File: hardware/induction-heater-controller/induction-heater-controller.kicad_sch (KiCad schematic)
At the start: 21 parts, among them IC1 THVD1449DR, J1 Conn_ARM_SWD_TagConnect_TC203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, J1 RJ12, J2 Screw_Terminal_01x02, SW1 SW_Push, SW3 SW_Push, U1 STM32G030F6Px, U2 NCP718xSN330

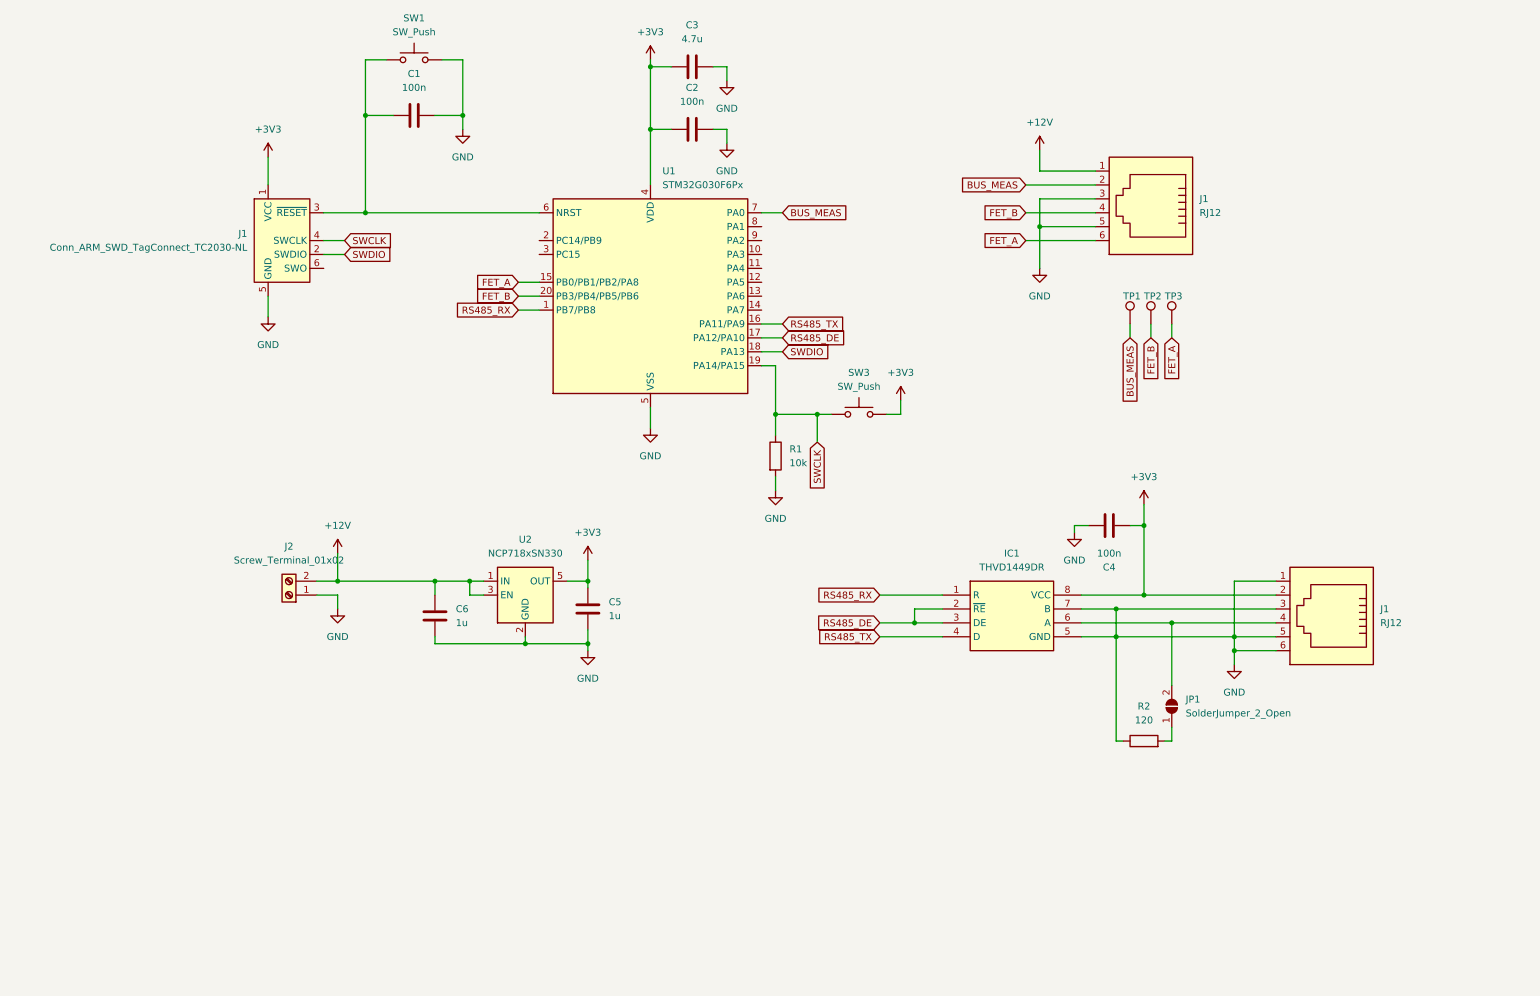
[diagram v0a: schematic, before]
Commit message: Finished board for controller
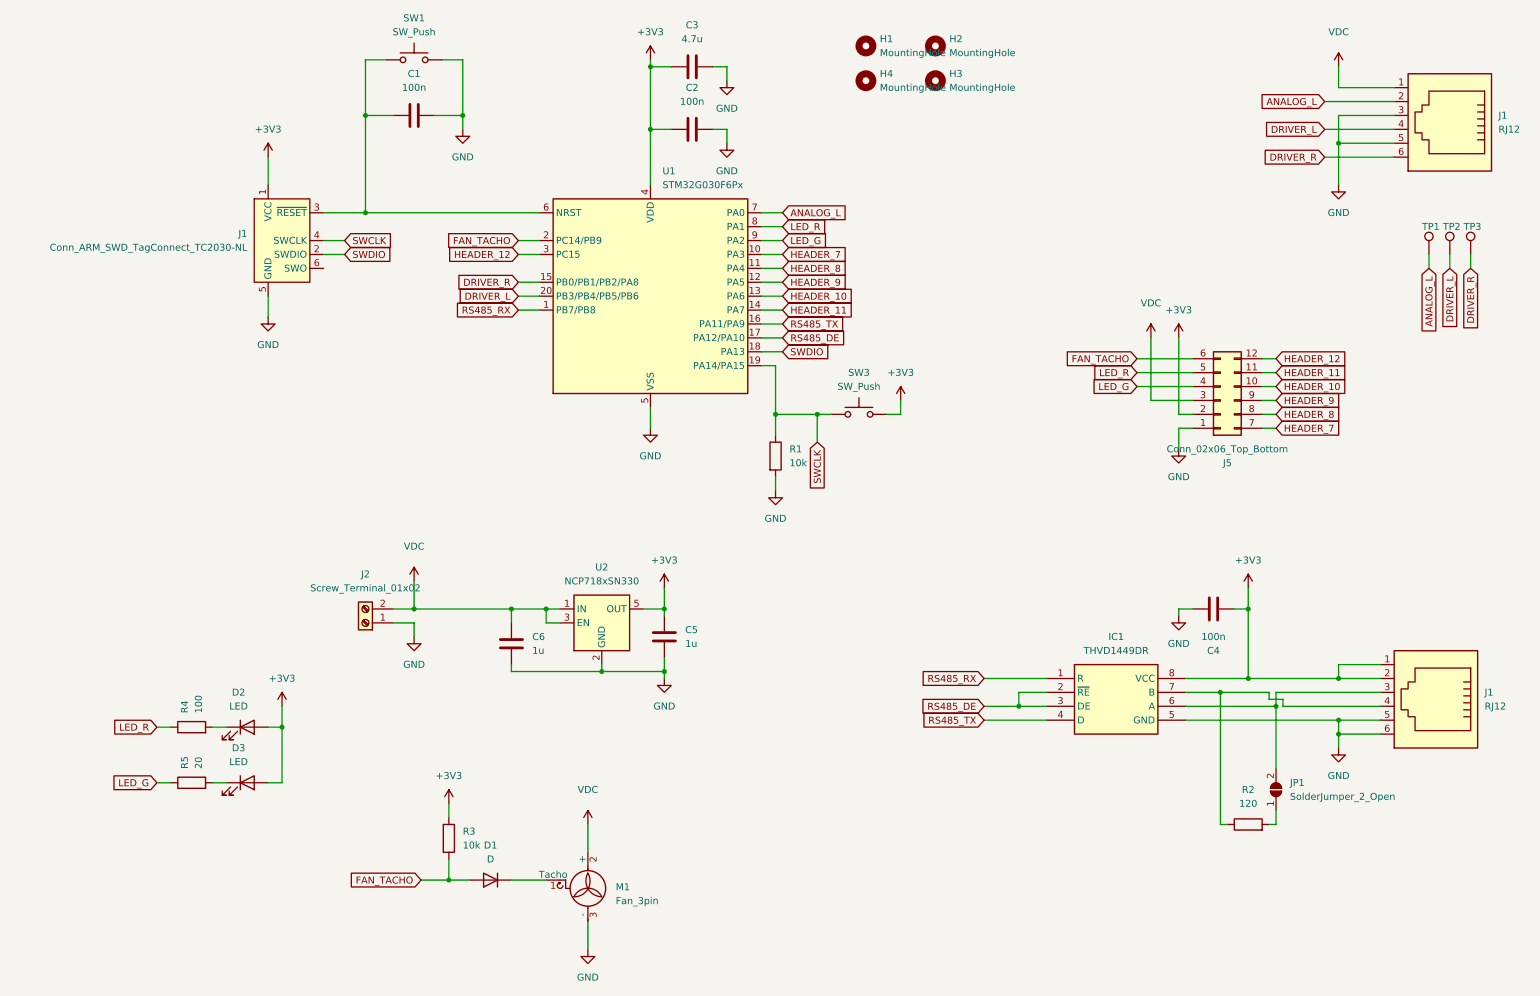
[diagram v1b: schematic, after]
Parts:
- added D1: D, Diode_SMD:D_SOD-523, symbol Device:D
- added D2, D3: LED, LED_SMD:LED_0805_2012Metric_Pad1.15x1.40mm_HandSolder, symbol Device:LED
- added H1, H2, H3, H4: MountingHole, Connector:Banana_Jack_1Pin, symbol Mechanical:MountingHole
- added J5: Conn_02x06_Top_Bottom, Connector_PinHeader_2.54mm:PinHeader_2x06_P2.54mm_Vertical, symbol Connector_Generic:Conn_02x06_Top_Bottom
- added M1: Fan_3pin, Connector:FanPinHeader_1x03_P2.54mm_Vertical, symbol Motor:Fan_3pin
- added R3: 10k, Resistor_SMD:R_0805_2012Metric_Pad1.20x1.40mm_HandSolder, symbol Device:R
- added R4: 100, Resistor_SMD:R_0805_2012Metric_Pad1.20x1.40mm_HandSolder, symbol Device:R
- added R5: 20, Resistor_SMD:R_0805_2012Metric_Pad1.20x1.40mm_HandSolder, symbol Device:R
- TP1, TP2, TP3: footprint (none) -> TestPoint:TestPoint_Pad_D1.5mm
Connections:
- net +3V3: now also J1.1, D2.2 (A), D3.2 (A), J5.2 (Pin_2), R3.1
- net GND: now also J5.1 (Pin_1), M1.3 (-); no longer IC1.7 (B), J1.1, J1.3, R2.1
- net at IC1.6 (A), JP1.2 (B): now also J1.3; no longer J1.4
- net HEADER_7: now reaches U1.10 (PA3)
- net HEADER_7: now also J5.7 (Pin_7)
- net HEADER_8: now reaches U1.11 (PA4)
- net HEADER_8: now also J5.8 (Pin_8)
- net HEADER_9: now reaches U1.12 (PA5)
- net HEADER_9: now also J5.9 (Pin_9)
- net HEADER_10: now reaches U1.13 (PA6)
- net HEADER_10: now also J5.10 (Pin_10)
- net HEADER_11: now reaches U1.14 (PA7)
- net HEADER_11: now also J5.11 (Pin_11)
- net FAN_TACHO: now reaches U1.2 (PC14/PB9)
- net FAN_TACHO: now also D1.2 (A), J5.6 (Pin_6), R3.2
- net HEADER_12: now reaches U1.3 (PC15)
- net HEADER_12: now also J5.12 (Pin_12)
- net LED_R: now reaches U1.8 (PA1)
- net LED_R: now also J5.5 (Pin_5), R4.1
- net LED_G: now reaches U1.9 (PA2)
- net LED_G: now also J5.4 (Pin_4), R5.1
- net +12V renamed VDC
- net VDC: now also J5.3 (Pin_3), M1.2 (+)
- net BUS_MEAS renamed ANALOG_L
- net FET_A renamed DRIVER_R
- net FET_B renamed DRIVER_L
- new net: D1.1 (K), M1.1 (Tacho)
- new net: D3.1 (K), R5.2
- new net: IC1.7 (B), J1.4, R2.1
- new net: D2.1 (K), R4.2
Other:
- moved on the sheet: C4, C5, C6, IC1, J1, J2, JP1, R2, TP1, TP2, TP3, U2

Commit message: Final components
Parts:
- C1, C2, C4: MPN (none) -> CL21B104KCFSFNG
- C3: MPN (none) -> CL21A475KAQNNNG
- C5, C6: MPN (none) -> CL21B105KAFNNNE
- IC1: MPN (none) -> THVD1449DR
- J5: MPN (none) -> 67997-212HLF
- R1, R3: MPN (none) -> RC0805JR-1010KL
- R2: MPN (none) -> RC0805FR-07120RL
- R4: MPN (none) -> RC0805JR-10100RL
- R5: MPN (none) -> RC0805FR-0720RL
- U1: MPN (none) -> STM32G030F6P6TR
- U2: MPN (none) -> NCP718ASN330T1G
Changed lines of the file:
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@@
+      (effects (font (size 1.27 1.27)) hide)
+    )
+    (property "MPN" "RC0805FR-0720RL" (at 41.91 154.94 0)
       (effects (font (size 1.27 1.27)) hide)
     )
@@
     (property "Manufacturer_Part_Number" "THVD1449DR" (at 219.71 930.81 0)
       (effects (font (size 1.27 1.27)) (justify left top) hide)
+    )
+    (property "MPN" "THVD1449DR" (at 198.12 135.89 0)
+      (effects (font (size 1.27 1.27)) hide)
     )
     (pin "1")
@@
       (effects (font (size 1.27 1.27)) hide)
     )
+    (property "MPN" "CL21B105KAFNNNE" (at 100.33 129.54 0)
+      (effects (font (size 1.27 1.27)) hide)
+    )
     (pin "1")
     (pin "2")
@@
     )
     (property "Datasheet" "https://www.st.com/resource/en/datasheet/stm32g030f6.pdf" (at 125.73 66.04 0)
+      (effects (font (size 1.27 1.27)) hide)
+    )
+    (property "MPN" "STM32G030F6P6TR" (at 125.73 66.04 0)
       (effects (font (size 1.27 1.27)) hide)
     )
@@
       (effects (font (size 1.27 1.27)) hide)
     )
+    (property "MPN" "CL21B104KCFSFNG" (at 228.6 123.19 90)
+      (effects (font (size 1.27 1.27)) hide)
+    )
     (pin "1")
     (pin "2")
@@
     )
     (property "Datasheet" "~" (at 229.87 85.09 0)
+      (effects (font (size 1.27 1.27)) hide)
+    )
+    (property "MPN" "67997-212HLF" (at 229.87 85.09 0)
       (effects (font (size 1.27 1.27)) hide)
     )
@@
       (effects (font (size 1.27 1.27)) hide)
     )
+    (property "MPN" "RC0805JR-1010KL" (at 148.59 95.25 0)
+      (effects (font (size 1.27 1.27)) hide)
+    )
     (pin "1")
     (pin "2")
@@
       (effects (font (size 1.27 1.27)) hide)
     )
+    (property "MPN" "CL21B105KAFNNNE" (at 128.27 128.27 0)
+      (effects (font (size 1.27 1.27)) hide)
+    )
     (pin "1")
     (pin "2")
@@
     )
     (property "Datasheet" "https://www.onsemi.com/pub/Collateral/NCP718-D.PDF" (at 116.84 113.03 0)
+      (effects (font (size 1.27 1.27)) hide)
+    )
+    (property "MPN" "NCP718ASN330T1G " (at 116.84 125.73 0)
       (effects (font (size 1.27 1.27)) hide)
     )
@@
       (effects (font (size 1.27 1.27)) hide)
     )
+    (property "MPN" "CL21B104KCFSFNG" (at 133.35 35.56 90)
+      (effects (font (size 1.27 1.27)) hide)
+    )
     (pin "1")
     (pin "2")
@@
       (effects (font (size 1.27 1.27)) hide)
     )
+    (property "MPN" "RC0805JR-10100RL" (at 41.91 144.78 0)
+      (effects (font (size 1.27 1.27)) hide)
+    )
     (pin "1")
     (pin "2")
@@
       (effects (font (size 1.27 1.27)) hide)
     )
+    (property "MPN" "RC0805FR-07120RL" (at 234.95 162.56 90)
+      (effects (font (size 1.27 1.27)) hide)
+    )
     (pin "1")
     (pin "2")
@@
       (effects (font (size 1.27 1.27)) hide)
     )
+    (property "MPN" "CL21A475KAQNNNG" (at 133.35 24.13 0)
+      (effects (font (size 1.27 1.27)) hide)
+    )
     (pin "1")
     (pin "2")
@@
     )
     (property "Datasheet" "~" (at 82.55 33.02 0)
+      (effects (font (size 1.27 1.27)) hide)
+    )
+    (property "MPN" "CL21B104KCFSFNG" (at 82.55 33.02 90)
       (effects (font (size 1.27 1.27)) hide)
     )
@@
       (effects (font (size 1.27 1.27)) hide)
     )
+    (property "MPN" "RC0805JR-1010KL" (at 88.9 165.1 0)
+      (effects (font (size 1.27 1.27)) hide)
+    )
